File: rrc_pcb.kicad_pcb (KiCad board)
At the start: 2 copper layers, 138.4 x 68.2 mm, 15 parts, among them J1 Conn_01x02_Male-Connector, J2 Conn_01x03_Male-Connector, J3 digital logic connection, U1 iridium9602, U2 Teensy4.1, U3 BN220-GPS, U4 ICM-20948, U5 MS5611, U6 logo, U7 Conn_01x02_Male-Connector

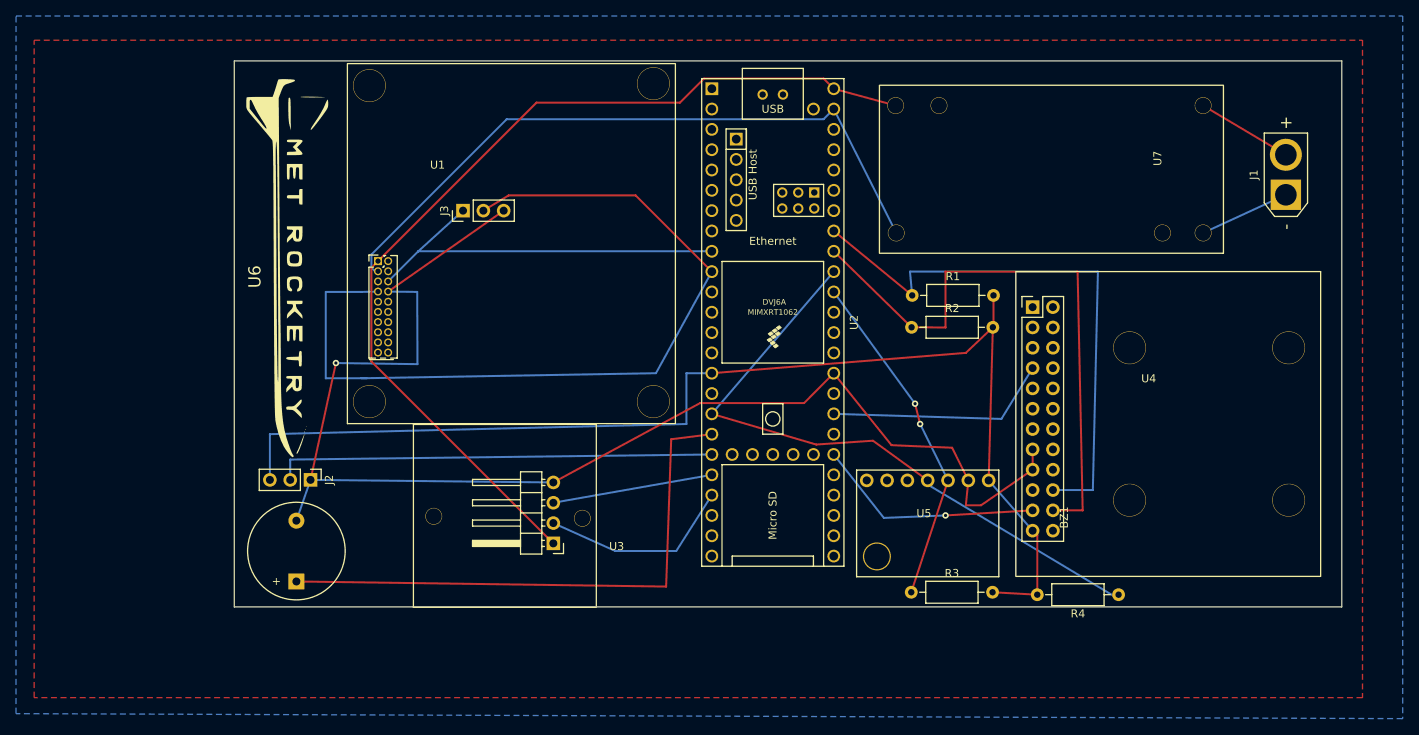
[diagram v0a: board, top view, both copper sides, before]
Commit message: Edit of PCB
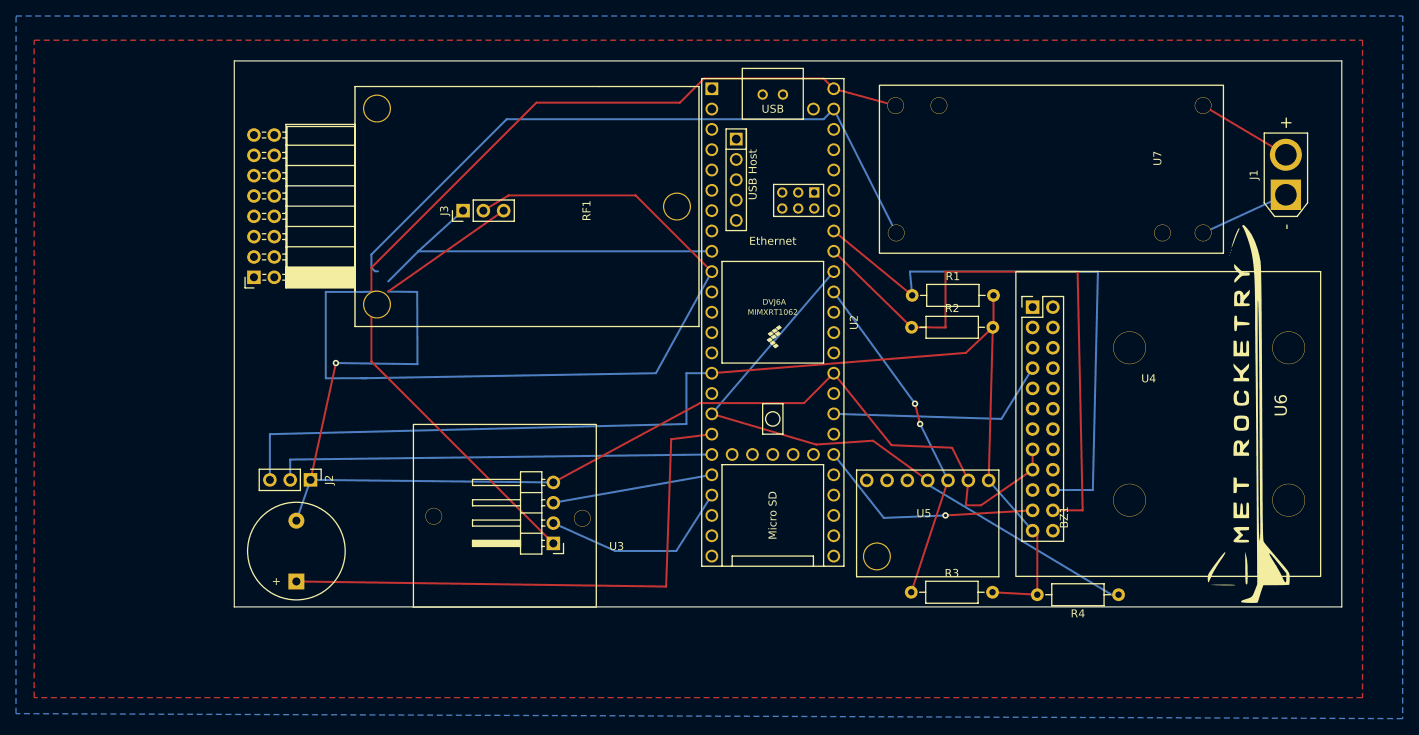
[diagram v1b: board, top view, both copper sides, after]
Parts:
- removed U1: iridium9602, iridium9602:iridium9602
- added RF1: RFD900+-RF_Module, rfd900+:RFD900+, F.Cu at (57.0, 23.9)
- U7: value Conn_01x02_Male-Connector -> voltReg
- moved U6 122.3 mm to (168.6, 67.7), turned to 90 degrees
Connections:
- U4 pad 24: unconnected-(U4-Pad24) -> VCC
